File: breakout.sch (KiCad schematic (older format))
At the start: 31 parts, among them CON1 SD_Card, CON2 USB-MICRO-AB, P2 CONN_01X40, P3 CONN_01X40, P4 CONN_01X40, P5 A-DF-09-A/KG-T4S, SW1 SW_PUSH

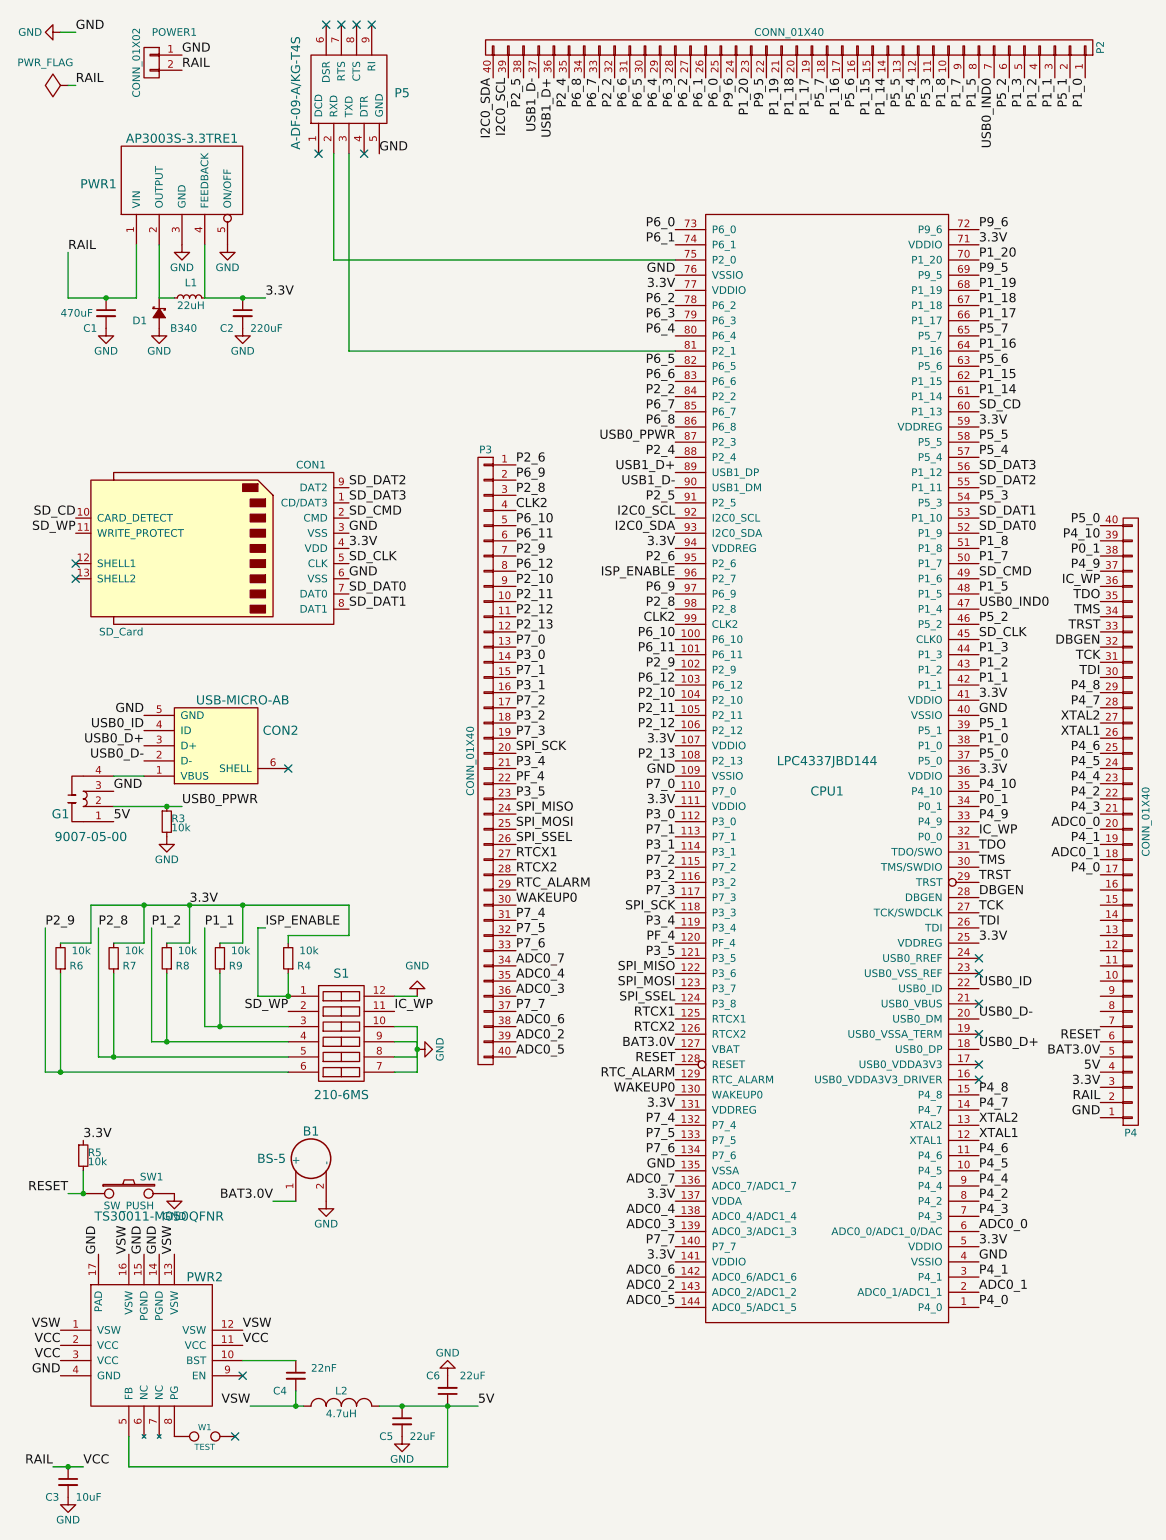
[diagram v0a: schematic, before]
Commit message: more decisions on component placement
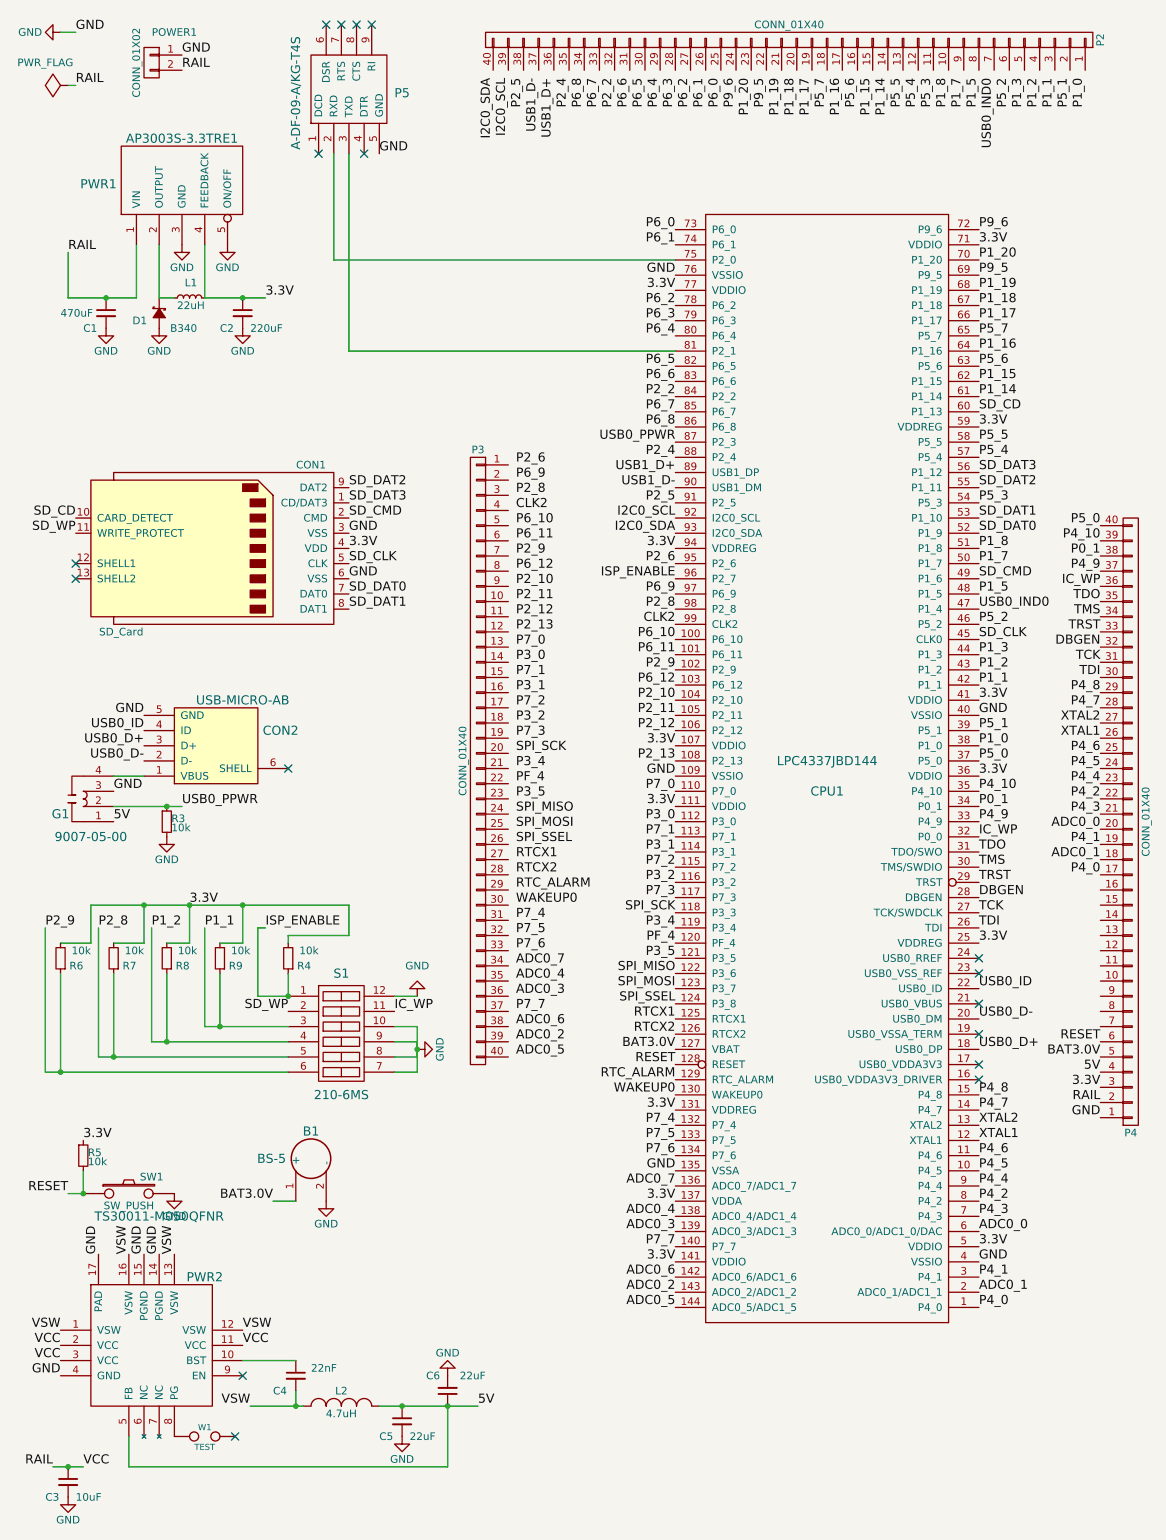
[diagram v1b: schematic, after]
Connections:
- net ADC0_2: no longer P3.39 (P39)
- net ADC0_3: no longer P3.36 (P36)
- net ADC0_4: no longer P3.35 (P35)
- net ADC0_5: no longer P3.40 (P40)
- net ADC0_6: no longer P3.38 (P38)
- net ADC0_7: no longer P3.34 (P34)
- net CLK2: no longer P3.4 (P4)
- net I2C0_SCL: no longer P2.39 (P39)
- net I2C0_SDA: no longer P2.40 (P40)
- net P1_0: no longer P2.1 (P1)
- net P1_1: no longer P2.3 (P3)
- net P1_14: no longer P2.14 (P14)
- net P1_15: no longer P2.15 (P15)
- net P1_16: no longer P2.17 (P17)
- net P1_17: no longer P2.19 (P19)
- net P1_18: no longer P2.20 (P20)
- net P1_19: no longer P2.21 (P21)
- net P1_2: no longer P2.4 (P4)
- net P1_20: no longer P2.23 (P23)
- net P1_3: no longer P2.5 (P5)
- net P1_5: no longer P2.8 (P8)
- net P1_7: no longer P2.9 (P9)
- net P1_8: no longer P2.10 (P10)
- net P2_10: no longer P3.9 (P9)
- net P2_11: no longer P3.10 (P10)
- net P2_12: no longer P3.11 (P11)
- net P2_13: no longer P3.12 (P12)
- net P2_2: no longer P2.32 (P32)
- net P2_4: no longer P2.35 (P35)
- net P2_5: no longer P2.38 (P38)
- net P2_6: no longer P3.1 (P1)
- net P2_8: no longer P3.3 (P3)
- net P2_9: no longer P3.7 (P7)
- net P3_0: no longer P3.14 (P14)
- net P3_1: no longer P3.16 (P16)
- net P3_2: no longer P3.18 (P18)
- net P3_4: no longer P3.21 (P21)
- net P3_5: no longer P3.23 (P23)
- net P5_1: no longer P2.2 (P2)
- net P5_2: no longer P2.6 (P6)
- net P5_3: no longer P2.11 (P11)
- net P5_4: no longer P2.12 (P12)
- net P5_5: no longer P2.13 (P13)
- net P5_6: no longer P2.16 (P16)
- net P5_7: no longer P2.18 (P18)
- net P6_0: no longer P2.25 (P25)
- net P6_1: no longer P2.26 (P26)
- net P6_10: no longer P3.5 (P5)
- net P6_11: no longer P3.6 (P6)
- net P6_12: no longer P3.8 (P8)
- net P6_2: no longer P2.27 (P27)
- net P6_3: no longer P2.28 (P28)
- net P6_4: no longer P2.29 (P29)
- net P6_5: no longer P2.30 (P30)
- net P6_6: no longer P2.31 (P31)
- net P6_7: no longer P2.33 (P33)
- net P6_8: no longer P2.34 (P34)
- net P6_9: no longer P3.2 (P2)
- net P7_0: no longer P3.13 (P13)
- net P7_1: no longer P3.15 (P15)
- net P7_2: no longer P3.17 (P17)
- net P7_3: no longer P3.19 (P19)
- net P7_4: no longer P3.31 (P31)
- net P7_5: no longer P3.32 (P32)
- net P7_6: no longer P3.33 (P33)
- net P7_7: no longer P3.37 (P37)
- net P9_5: no longer P2.22 (P22)
- net P9_6: no longer P2.24 (P24)
- net PF_4: no longer P3.22 (P22)
- net RTCX1: no longer P3.27 (P27)
- net RTCX2: no longer P3.28 (P28)
- net RTC_ALARM: no longer P3.29 (P29)
- net SPI_MISO: no longer P3.24 (P24)
- net SPI_MOSI: no longer P3.25 (P25)
- net SPI_SCK: no longer P3.20 (P20)
- net SPI_SSEL: no longer P3.26 (P26)
- net USB0_IND0: no longer P2.7 (P7)
- net USB1_D+: no longer P2.36 (P36)
- net USB1_D-: no longer P2.37 (P37)
- net WAKEUP0: no longer P3.30 (P30)
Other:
- moved on the sheet: P2, P3
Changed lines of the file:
@@
 L CONN_01X40 P3
 U 1 1 5614BAE0
-P 3600 5400
-F 0 "P3" H 3600 7450 50  0000 C CNN
-F 1 "CONN_01X40" V 3700 5400 50  0000 C CNN
-F 2 "Socket_Strips:Socket_Strip_Straight_1x40" H 3600 5400 60  0001 C CNN
-F 3 "" H 3600 5400 60  0000 C CNN
-	1    3600 5400
+P 3550 5400
+F 0 "P3" H 3550 7450 50  0000 C CNN
+F 1 "CONN_01X40" V 3650 5400 50  0000 C CNN
+F 2 "Socket_Strips:Socket_Strip_Straight_1x40" H 3550 5400 60  0001 C CNN
+F 3 "" H 3550 5400 60  0000 C CNN
+	1    3550 5400
 	-1   0    0    -1
 $EndComp
@@
 L CONN_01X40 P2
 U 1 1 5614BB79
-P 5600 700
-F 0 "P2" H 5600 2750 50  0000 C CNN
-F 1 "CONN_01X40" V 5700 700 50  0000 C CNN
-F 2 "Socket_Strips:Socket_Strip_Straight_1x40" H 5600 700 60  0001 C CNN
-F 3 "" H 5600 700 60  0000 C CNN
-	1    5600 700
+P 5600 650
+F 0 "P2" H 5600 2700 50  0000 C CNN
+F 1 "CONN_01X40" V 5700 650 50  0000 C CNN
+F 2 "Socket_Strips:Socket_Strip_Straight_1x40" H 5600 650 60  0001 C CNN
+F 3 "" H 5600 650 60  0000 C CNN
+	1    5600 650
 	0    1    -1   0
 $EndComp
